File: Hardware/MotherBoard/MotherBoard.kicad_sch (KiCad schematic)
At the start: 16 parts, among them J1 POWER, J10 I/O_PWR, J2 I/O0, J5 I/O1, J6 EXTRN_CLCK, U1 AMS1117-5.0

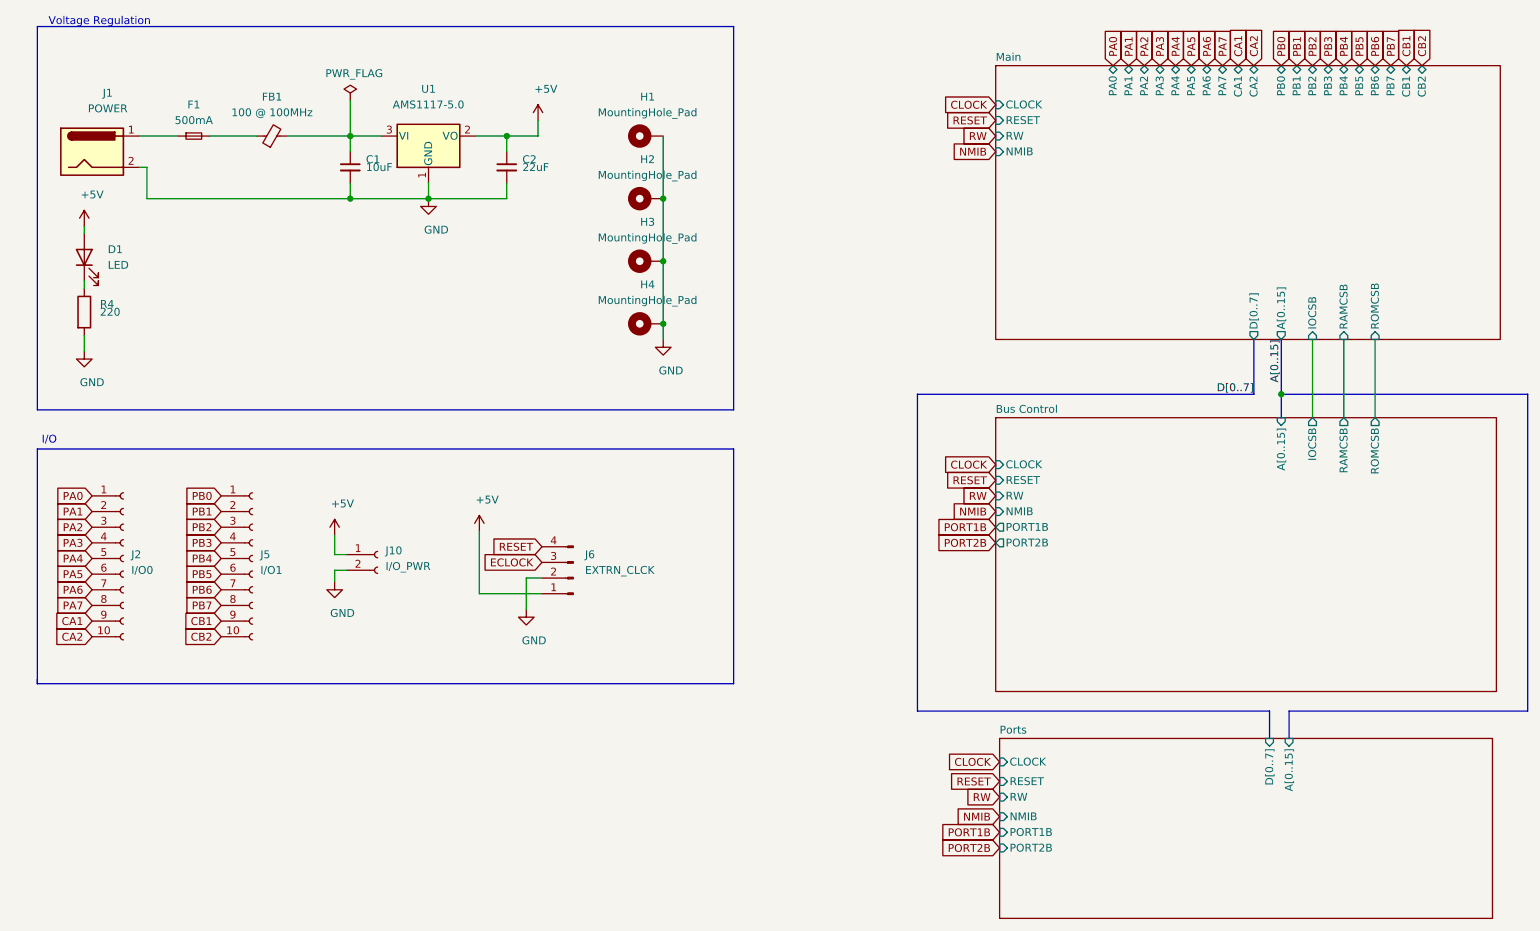
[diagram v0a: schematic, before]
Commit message: Fix
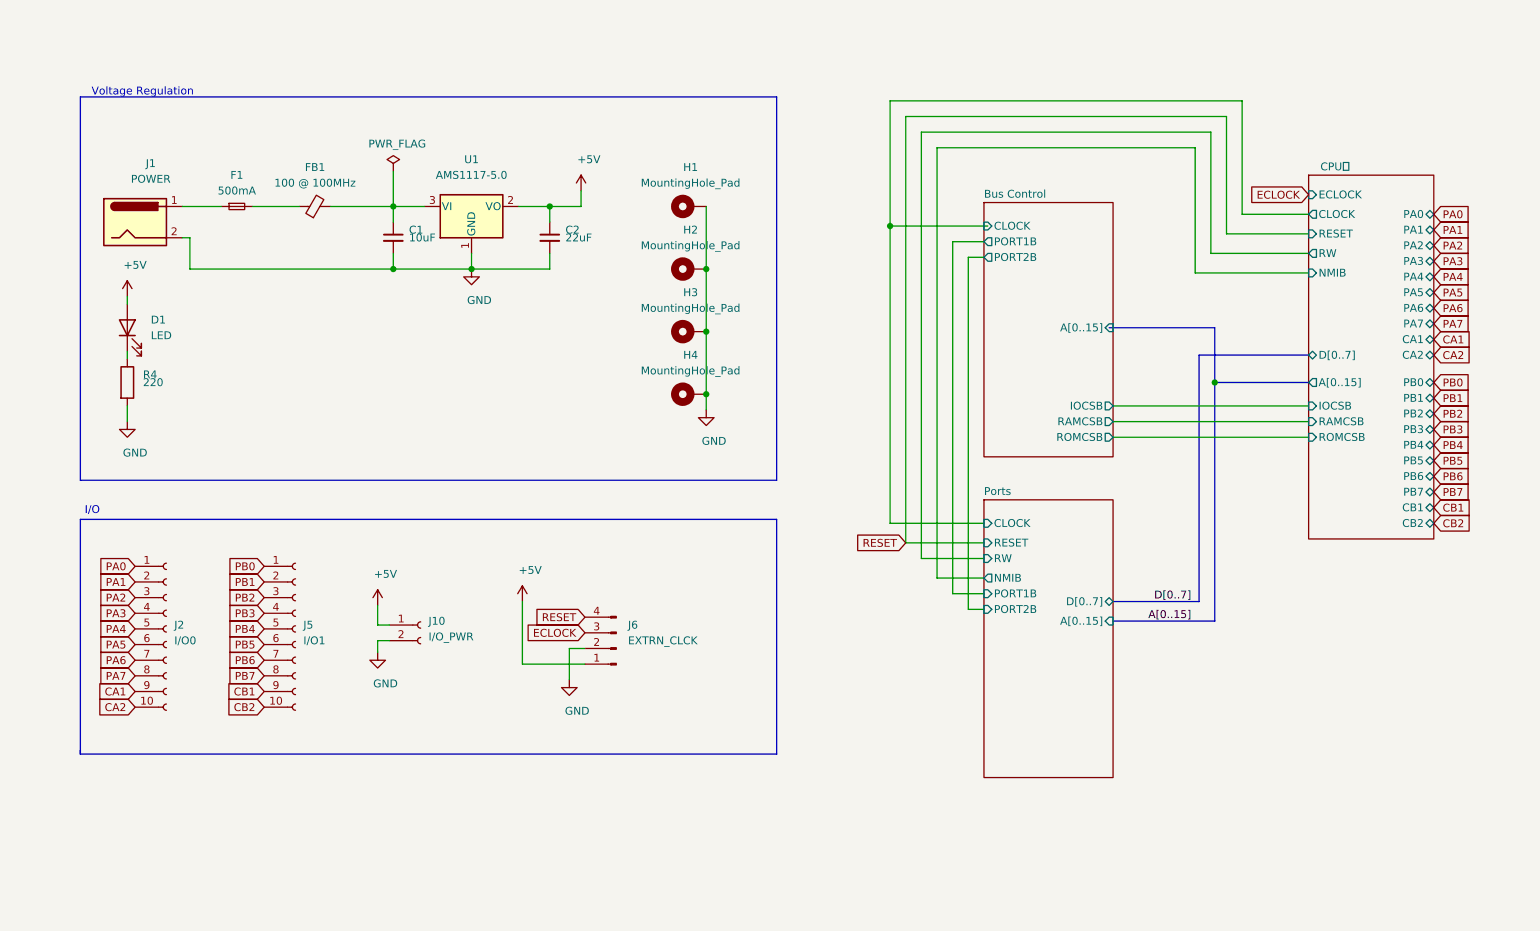
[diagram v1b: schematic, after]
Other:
- sheet Main renamed CPU 
- sheet Bus Control ports: added none; removed NMIB, RESET, RW
- sheet CPU  ports: added ECLOCK; removed none
- moved on the sheet: C1, C2, D1, F1, FB1, H1, H2, H3, H4, J1, J10, J2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
